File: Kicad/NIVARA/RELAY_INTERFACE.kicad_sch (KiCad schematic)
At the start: 3 parts, among them K1 G2RL-1, K2 G2RL-1

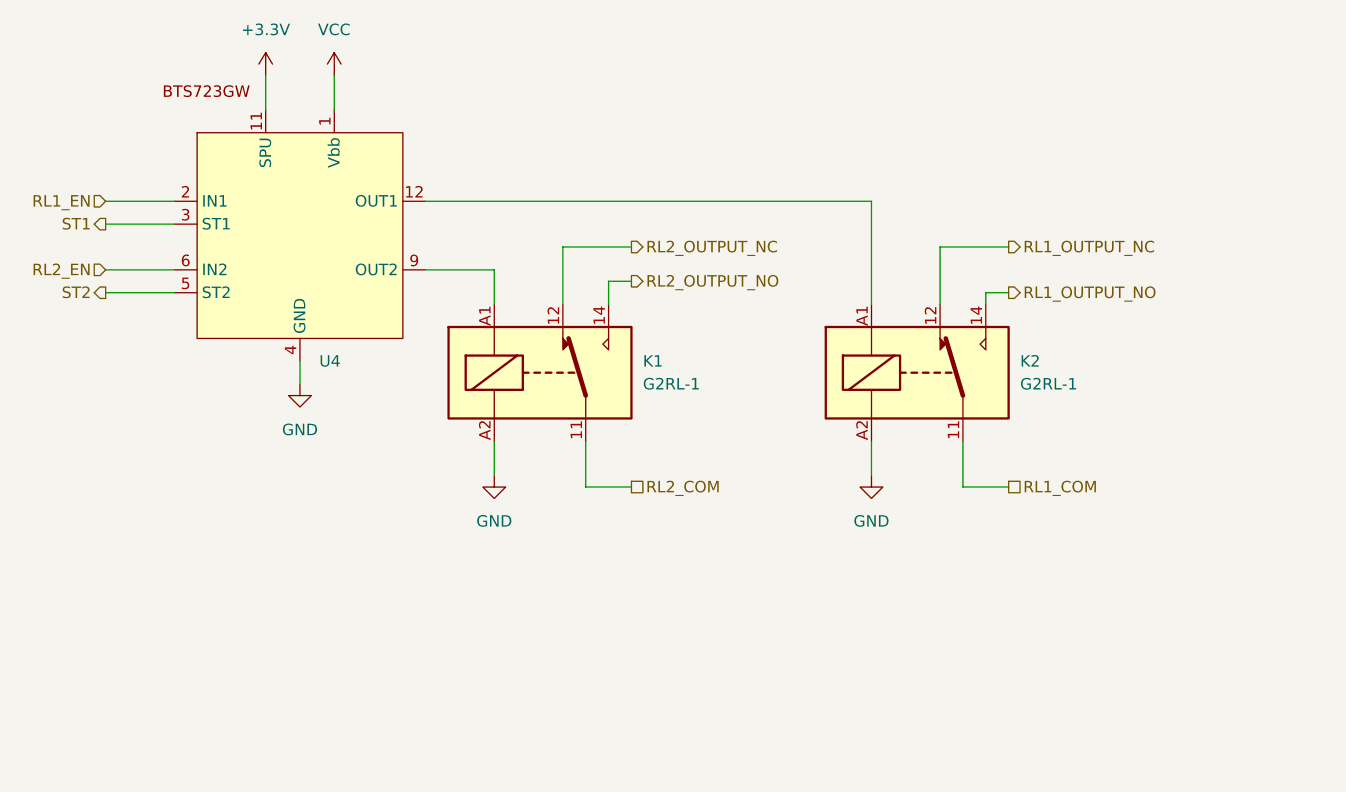
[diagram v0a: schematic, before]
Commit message: ZZZ
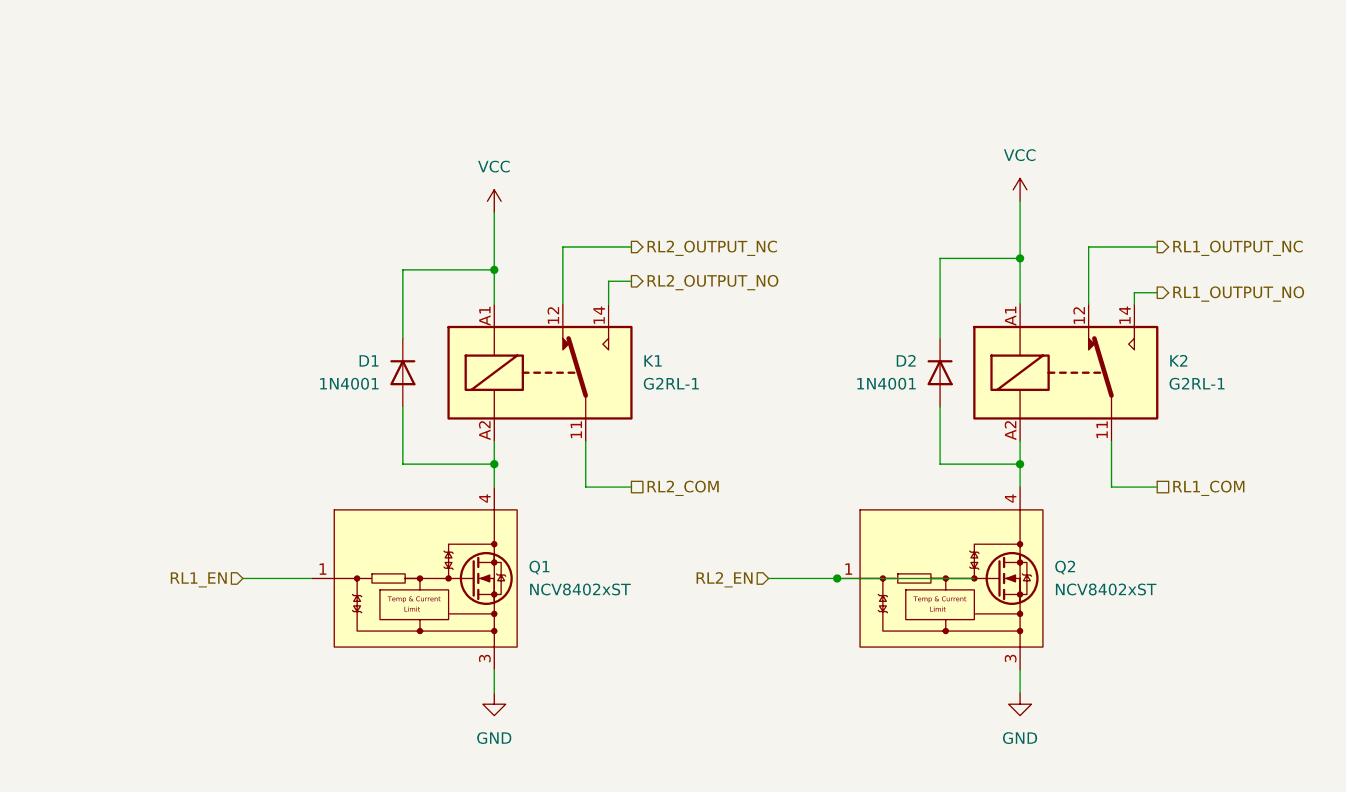
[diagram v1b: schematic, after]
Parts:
- removed U4: ~, Riqi_Parts:SOIC127P600X172-14N, symbol Riqi_Parts:BTS723GW
- added D1, D2: 1N4001, Diode_SMD:D_SMA, symbol Diode:1N4001
- added Q1, Q2: NCV8402xST, Package_TO_SOT_SMD:SOT-223, symbol Driver_FET:NCV8402xST
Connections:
- net GND: now also Q1.3 (S), Q2.3 (S); no longer K1.A2, K2.A2
- net RL1_EN: now also Q1.1 (G)
- net RL2_EN: now also Q2.1 (G)
- net VCC: now also K1.A1, K2.A1, D1.1 (K), D2.1 (K)
- new net: D1.2 (A), K1.A2, Q1.2 (D), Q1.4 (D)
- new net: D2.2 (A), K2.A2, Q2.2 (D), Q2.4 (D)
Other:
- moved on the sheet: K2

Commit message: .
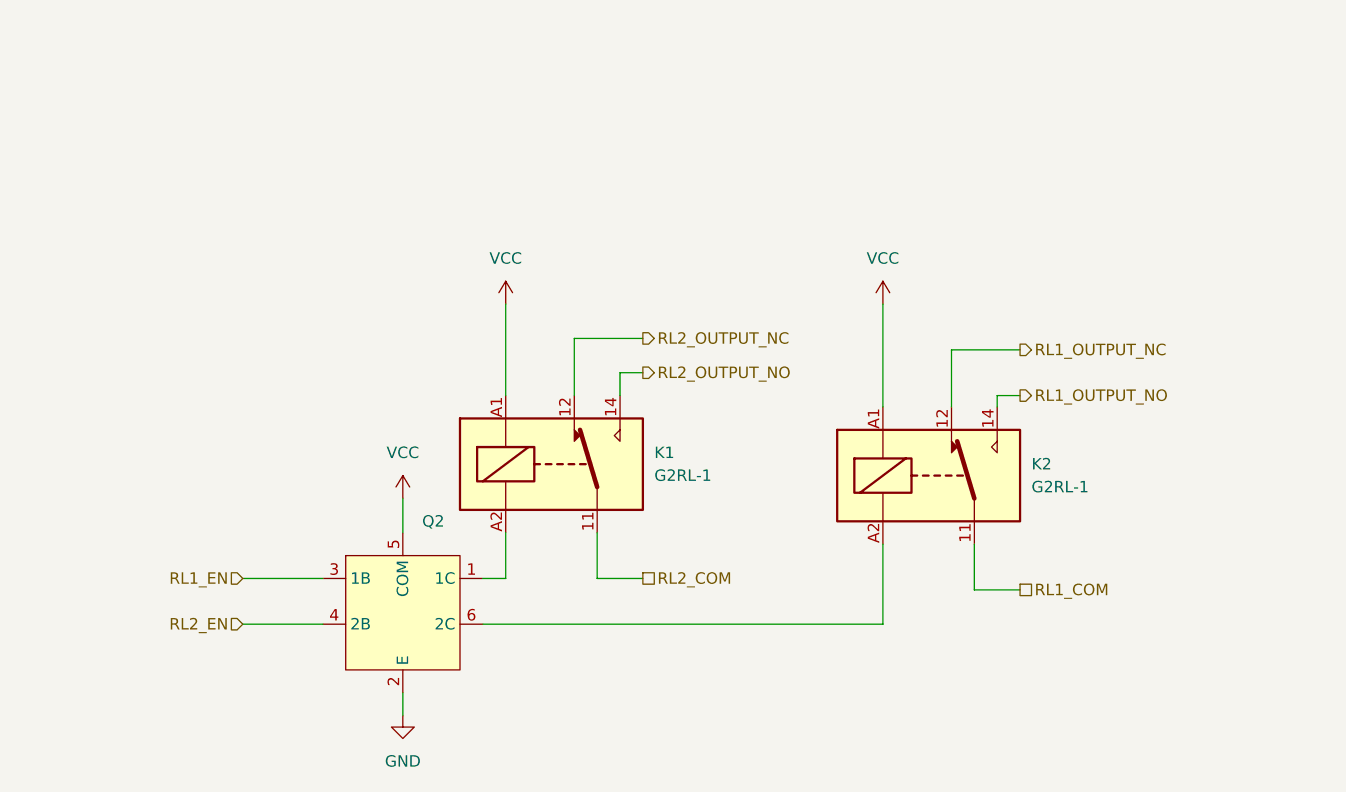
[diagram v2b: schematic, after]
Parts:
- removed D1, D2: 1N4001, Diode_SMD:D_SMA, symbol Diode:1N4001
- removed Q1, Q2: NCV8402xST, Package_TO_SOT_SMD:SOT-223, symbol Driver_FET:NCV8402xST
- added Q2: ~, symbol Riqi_Parts:LANKE LK1802
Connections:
- net GND: now also Q2.2 (E)
- net RL1_EN: now also Q2.3 (1B)
- net RL2_EN: now also Q2.4 (2B)
- net VCC: now also Q2.5 (COM)
- net at K1.A2: now also Q2.1 (1C)
- net at K2.A2: now also Q2.6 (2C)
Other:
- moved on the sheet: K1, K2

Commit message: Debí de enrutar antes :C
tengo sueño
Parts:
- Q2: footprint (none) -> Package_TO_SOT_SMD:SOT-363_SC-70-6
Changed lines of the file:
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@@
 			)
 		)
-		(property "Footprint" ""
+		(property "Footprint" "Package_TO_SOT_SMD:SOT-363_SC-70-6"
 			(at 105.41 105.41 0)
 			(effects
